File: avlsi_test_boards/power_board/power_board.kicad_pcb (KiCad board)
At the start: 4 copper layers, 105 parts, among them J1 PJ-102AH, J2 PJ-102AH, J3 Conn_02x07_Top_Bottom, J5 Conn_02x20_Odd_Even, J6 Conn_02x20_Odd_Even, J7 Conn_02x20_Odd_Even, J8 Conn_02x20_Odd_Even, J9 Conn_02x07_Top_Bottom, U1 TLV1117LV18DCYR, U11 SN74LVC16T245DLR, U12 SN74LVC16T245DLR, U13 SN74LVC16T245DLR, U14 SN74LVC16T245DLR, U15 DS04-254-2-04BK-SMT, U17 SN74LVC16T245DLR, U18 SN74LVC16T245DLR, U19 SN74LVC16T245DLR, U20 74HC4051D_653, U3 TLV1117LV25DCYR, U4 TLV1117LV33DCYR, U5 TLV1117LV18DCYR, U6 TLV75709PDBV, U7 TLV1117LV25DCYR, U8 TLV1117LV33DCYR

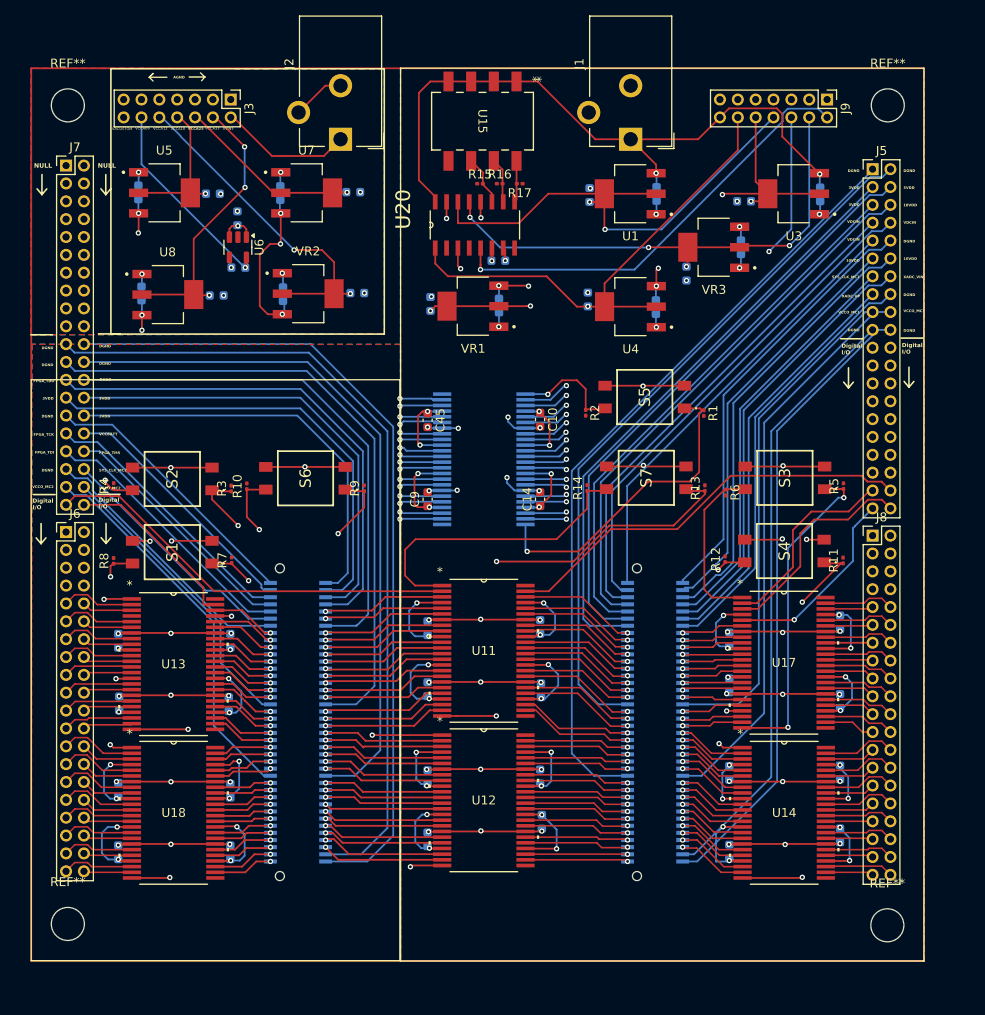
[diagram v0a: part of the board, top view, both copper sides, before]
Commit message: more changes
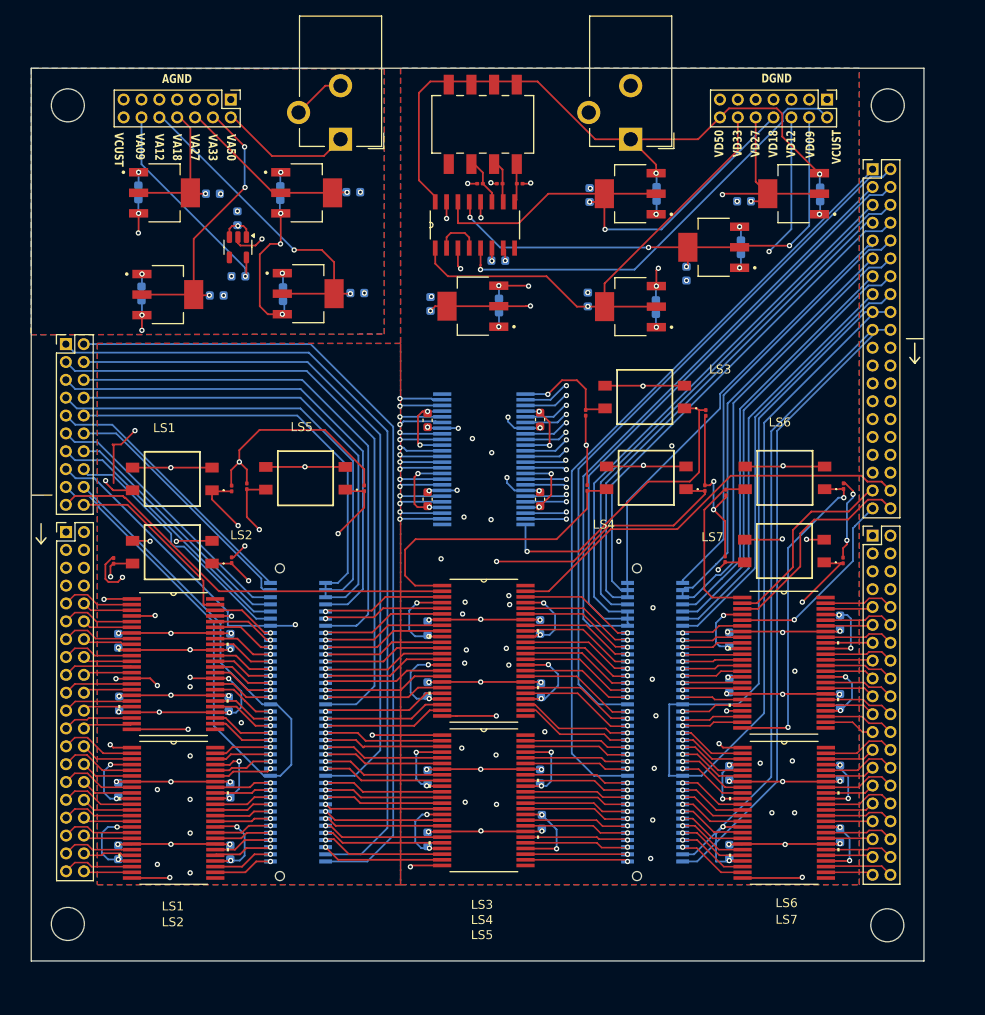
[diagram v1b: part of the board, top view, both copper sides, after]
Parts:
- removed J7: Conn_02x20_Odd_Even, Connector_PinHeader_2.00mm:PinHeader_2x20_P2.00mm_Vertical
- removed R4: 4.7k, Resistor_SMD:R_0201_0603Metric
- added J4: Conn_02x10_Odd_Even, Connector_PinHeader_2.00mm:PinHeader_2x10_P2.00mm_Vertical, F.Cu at (103.4, 63.1)
- moved C42 0.98 mm to (122.7, 55.5)
- moved U15 0.36 mm to (150.1, 38.5)
- moved R1 0.22 mm to (175.1, 70.9)
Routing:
- net DGND: track 1122.4 -> 1233.2 mm, vias 66 -> 123
- net /pin_header/VCCO_MC2: track 76.6 -> 87.7 mm
- net /pin_header/VCCO_MC1: track 120.8 -> 131.8 mm
- net DVIN5: track 127.1 -> 133.2 mm
- net /digital_power_converters/NULL: track 0.00 -> 5.35 mm
- net ADGND: track 12.2 -> 16.0 mm, vias 10 -> 11
- net /pin_header/VDCIN: track 161.9 -> 164.7 mm
- net /VCCA09: track 23.2 -> 25.1 mm
- net /pin_header/33VDD: track 194.9 -> 196.6 mm
- net /pin_header/3VDD: track 150.9 -> 152.5 mm
- net /pin_header/10VDD: track 95.9 -> 96.7 mm
- net /pin_header/HB8: track 45.4 -> 46.2 mm
- net /pin_header/SYS_CLK_MC2: track 27.8 -> 28.6 mm
- net /pin_header/HA2: track 40.8 -> 41.3 mm
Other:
- board outline added: 100 x 100 mm
- board text added: "LS1"
- board text added: "LS2"
- board text added: "LS3"
- board text added: "LS4"
- board text added: "LS5"
- board text added: "LS6"
- board text added: "LS7"
- board text added: "VA09"
- board text added: "VA12"
- board text added: "VA18"
- board text added: "VA27"
- board text added: "VA33"
- board text added: "VA50"
- board text added: "VCUST"
- board text added: "VD09"
- board text added: "VD12"
- board text added: "VD18"
- board text added: "VD27"
- board text added: "VD33"
- board text added: "VD50"
- board text removed: "10VDD"
- board text removed: "18VDD"
- board text removed: "3VDD"
- board text removed: "AVIN5"
- board text removed: "Digital I/O"
- board text removed: "FPGA_TCK"
- board text removed: "FPGA_TDI"
- board text removed: "FPGA_TDO"
- board text removed: "FPGA_TMS"
- board text removed: "NULL"
- board text removed: "SYS_CLK_MC1"
- board text removed: "SYS_CLK_MC2"
- board text removed: "VACUSTOM"
- board text removed: "VCCA09"
- board text removed: "VCCA12"
- board text removed: "VCCA18"
- board text removed: "VCCA25"
- board text removed: "VCCA33"
- board text removed: "VCCBATT"
- board text removed: "VCCO_MC1"
- board text removed: "VCCO_MC2"
- board text removed: "VDCIN"
- board text removed: "XADC_VIN"
- board text removed: "XADC_VP"
